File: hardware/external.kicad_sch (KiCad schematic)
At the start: 7 parts

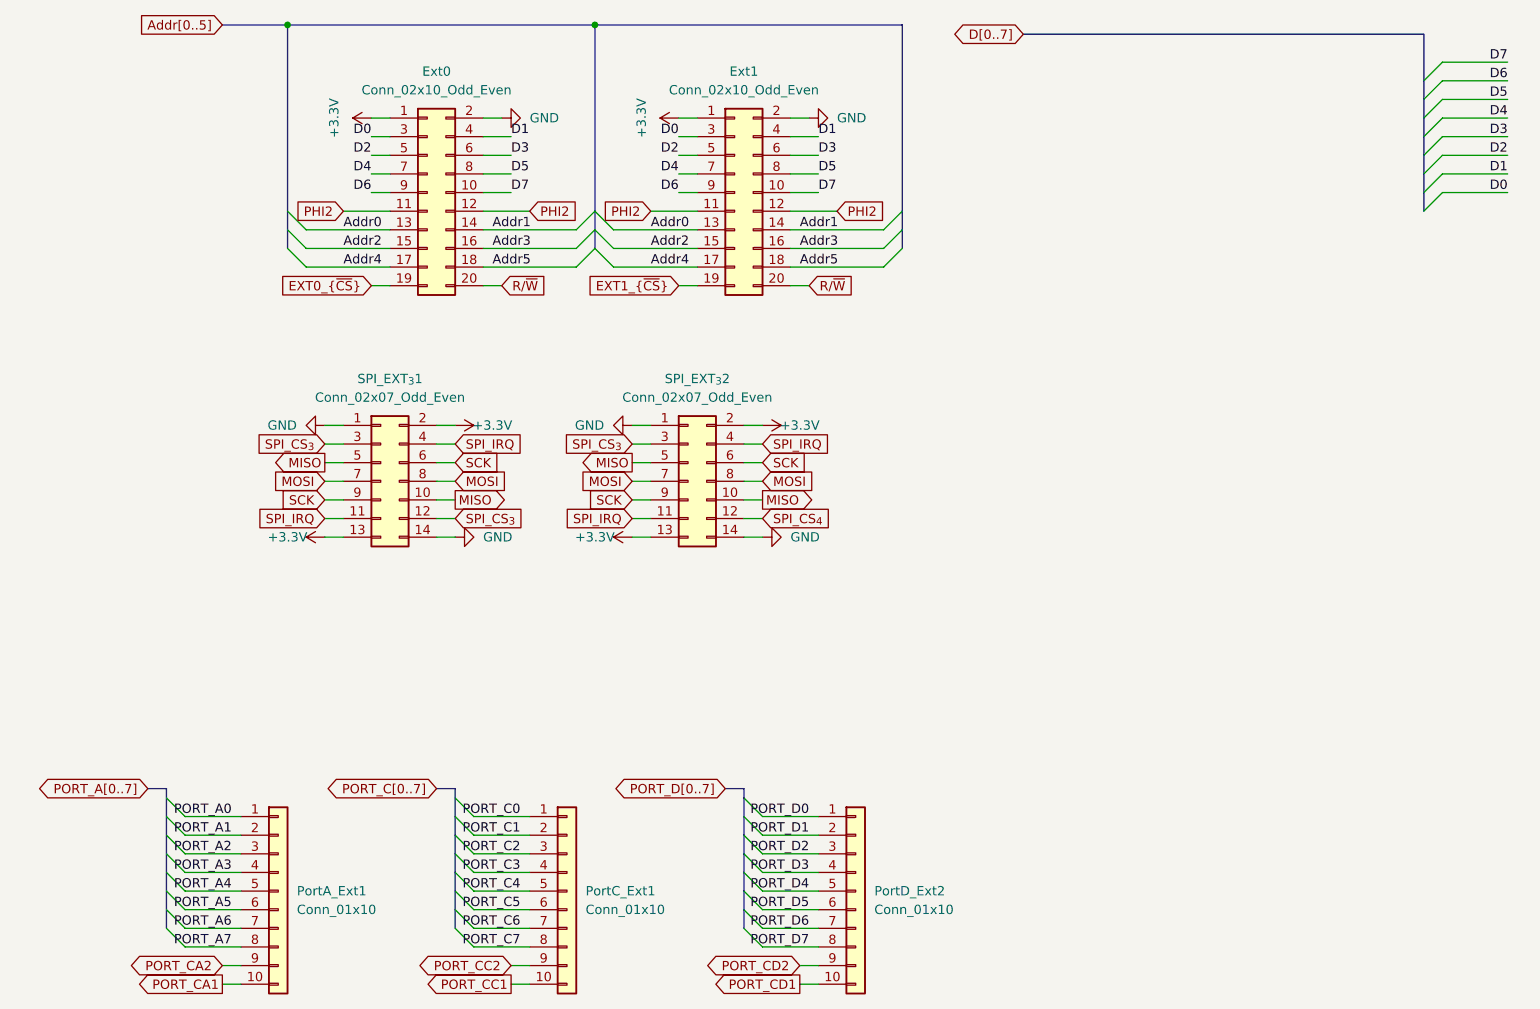
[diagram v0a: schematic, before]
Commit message: Fixes and addres fix adding VDA AND VPA
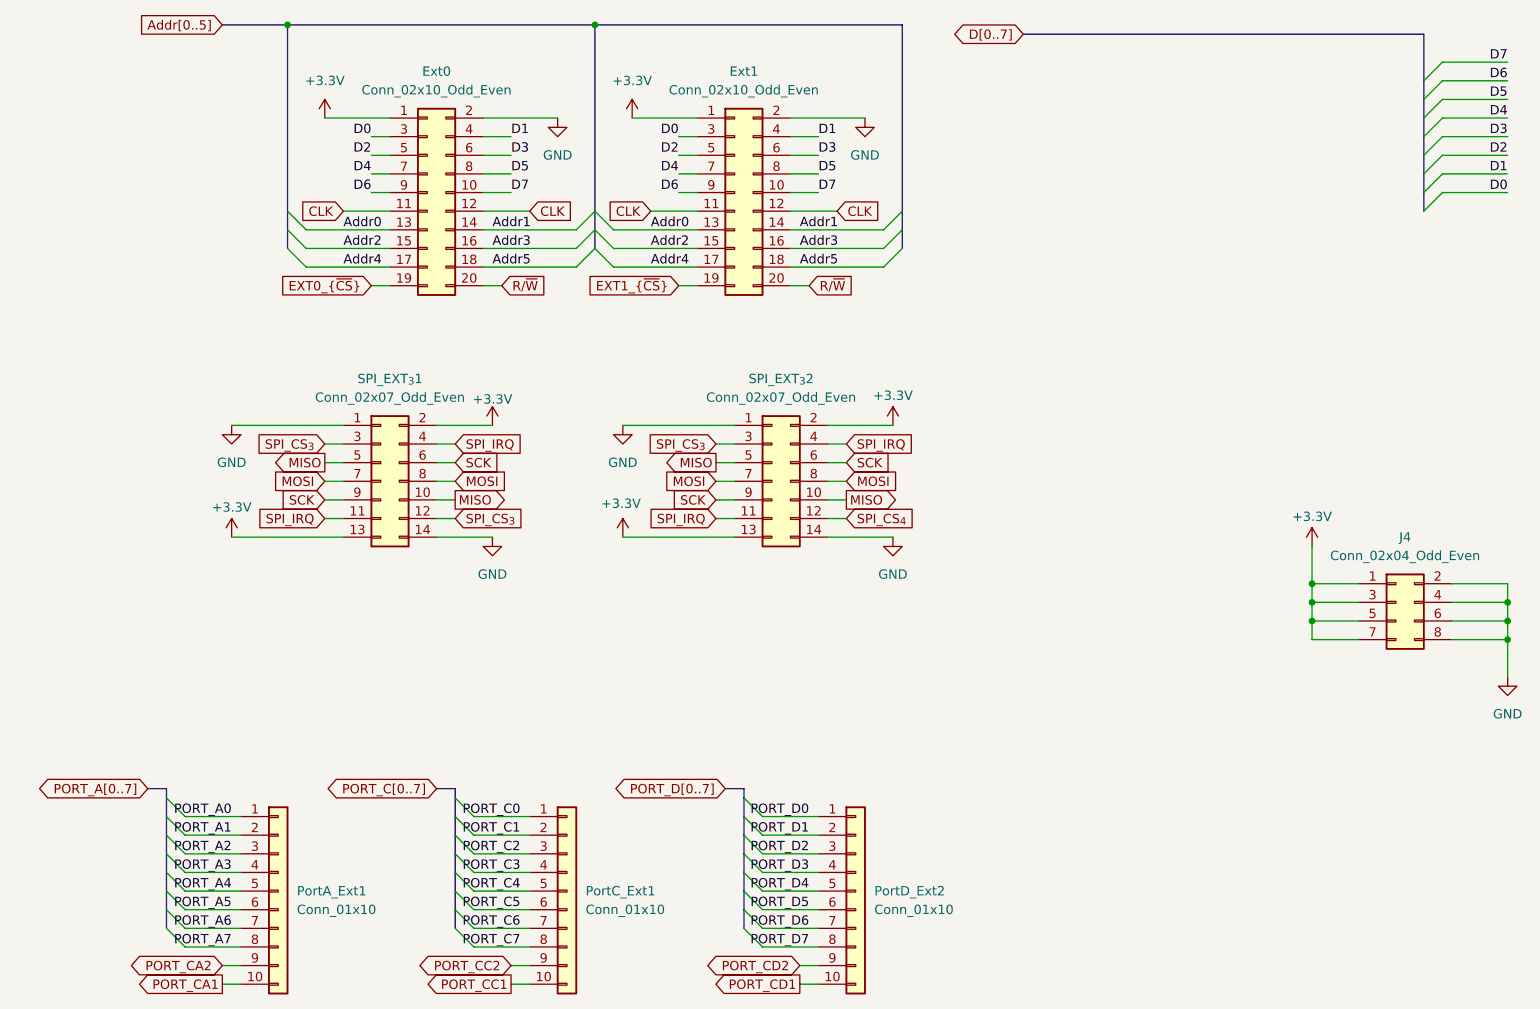
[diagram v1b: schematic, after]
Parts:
- added J4: Conn_02x04_Odd_Even, Connector_PinHeader_2.54mm:PinHeader_2x04_P2.54mm_Vertical, symbol Connector_Generic:Conn_02x04_Odd_Even
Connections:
- net +3.3V: now also J4.1 (Pin_1), J4.3 (Pin_3), J4.5 (Pin_5), J4.7 (Pin_7)
- net GND: now also J4.2 (Pin_2), J4.4 (Pin_4), J4.6 (Pin_6), J4.8 (Pin_8)
- net PHI2 renamed CLK
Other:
- moved on the sheet: SPI_EXT_{3}2
